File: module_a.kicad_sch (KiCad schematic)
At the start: 34 parts, among them J1 RS232, J2 Ethernet, J3 Micro_SD_Card_Det2, U1 MAX3232, U18 74LVC1G07, U2 SN74AHC123A, U3 TPD4EUSB30, U4 TPD4EUSB30, U5 TPS2553

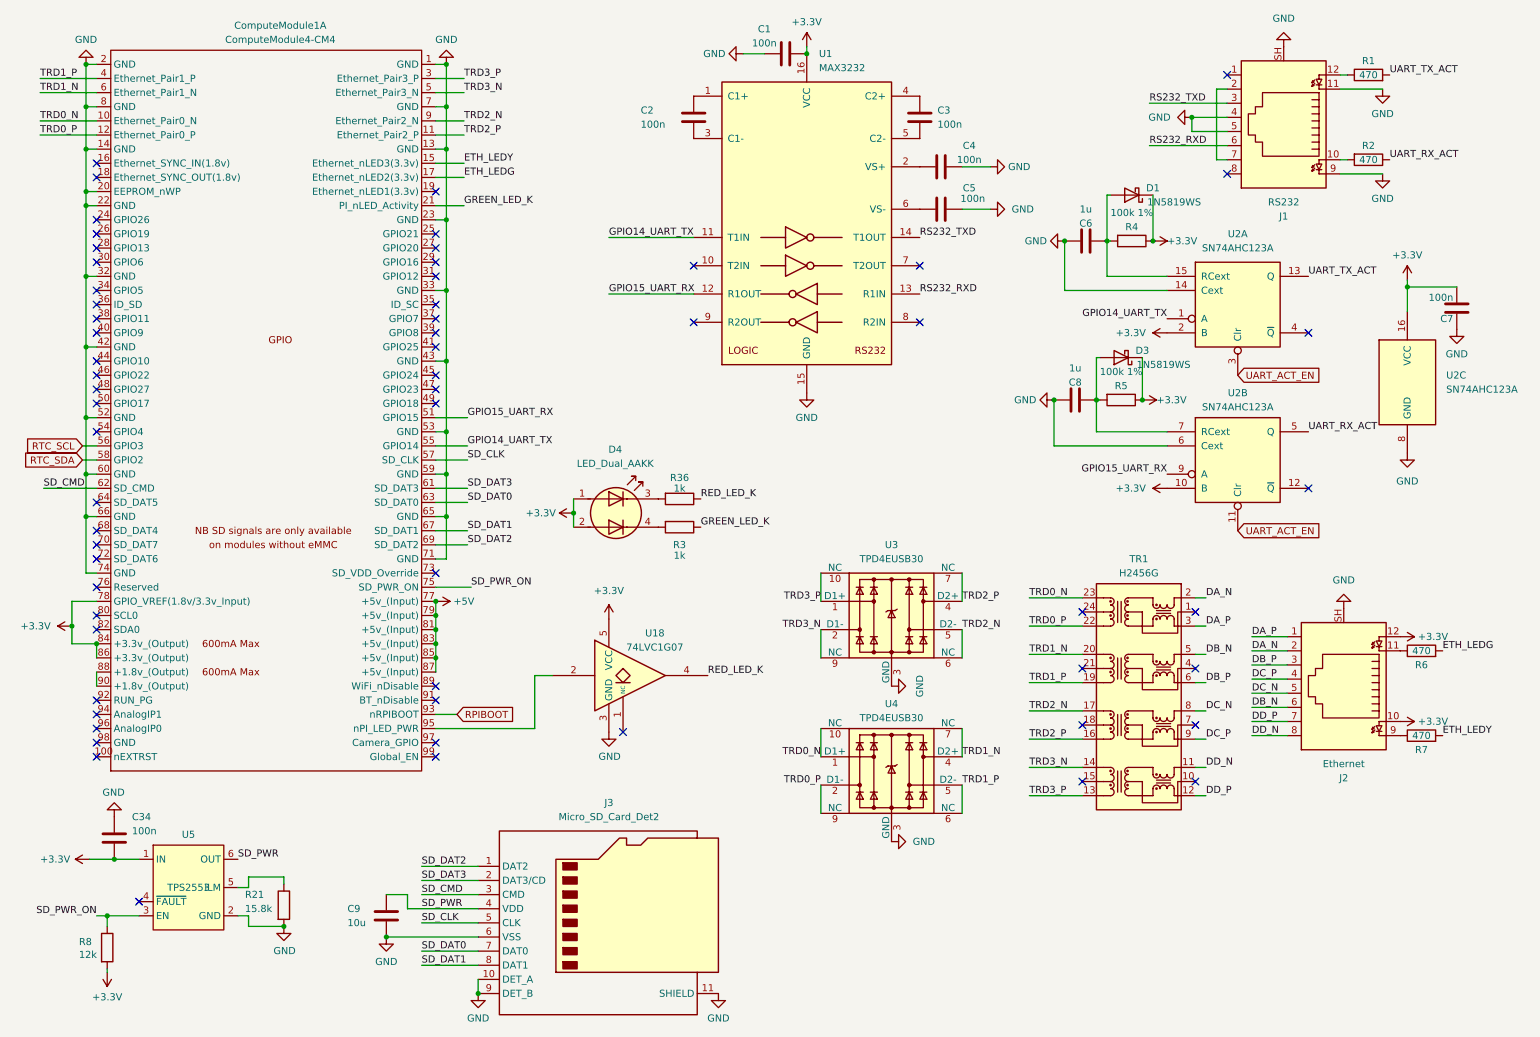
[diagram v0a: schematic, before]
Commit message: wip
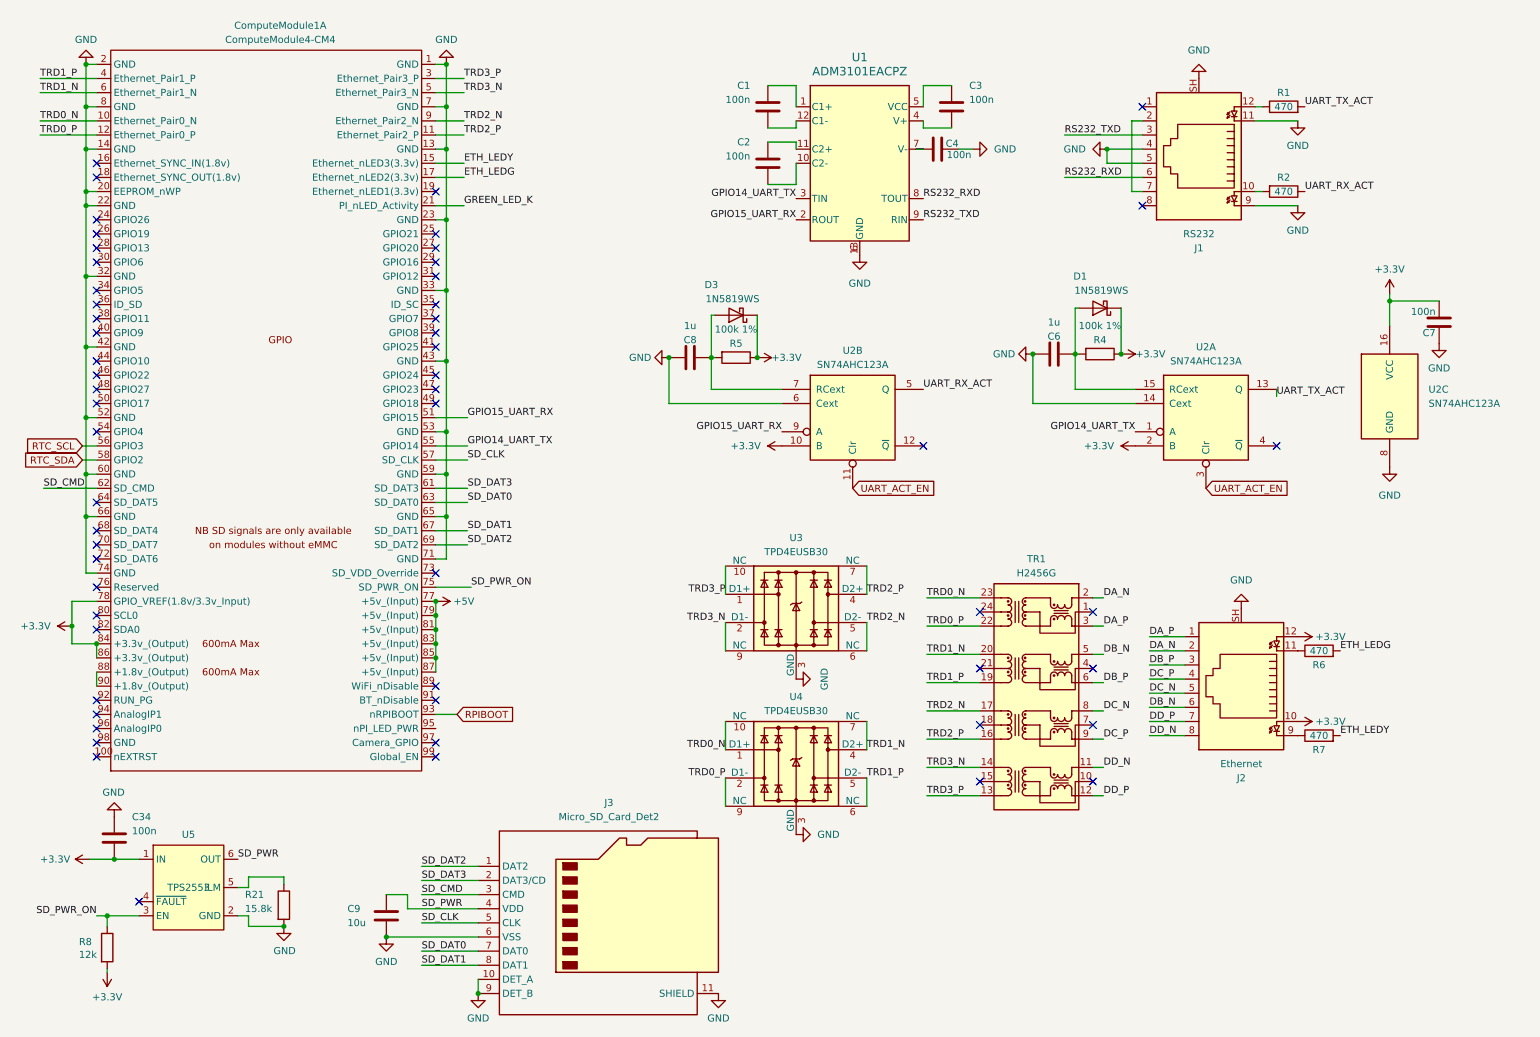
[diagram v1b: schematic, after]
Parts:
- removed C5: 100n, Capacitor_SMD:C_0402_1005Metric, symbol Device:C
- removed D4: LED_Dual_AAKK, PiCard:LED-ARRAY-SMD_4P-L3.0-W1.5-L-FD, symbol Device:LED_Dual_AAKK
- removed R3, R36: 1k, Resistor_SMD:R_0402_1005Metric, symbol Device:R
- removed U1: MAX3232, Package_SO:TSSOP-16_4.4x5mm_P0.65mm, symbol Interface_UART:MAX3232
- removed U18: 74LVC1G07, Package_TO_SOT_SMD:SOT-353_SC-70-5, symbol 74xGxx:74LVC1G07
- added U1: ADM3101EACPZ, PiCard:LFCSP-12-1EP_3x3mm_P0.5mm_EP1.3x1.3mm, symbol PiCard:ADM3101EACPZ
- U2: footprint Package_SO:TSSOP-16_4.4x5mm_P0.65mm -> Package_DFN_QFN:DHVQFN-16-1EP_2.5x3.5mm_P0.5mm_EP1x2mm
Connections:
- net +3.3V: no longer C1.2
- net GND: now also U1.13 (GND), U1.6 (GND); no longer C1.1
- net GPIO14_UART_TX: now also U1.3 (TIN)
- net GPIO15_UART_RX: now also U1.2 (ROUT)
- net RS232_RXD: now also U1.8 (TOUT)
- net RS232_TXD: now also U1.9 (RIN)
- net at C2.1: now also U1.11 (C2+)
- net at C4.1: now also U1.7 (V-)
- net at C2.2: now also U1.10 (C2-)
- net at C3.1: now also U1.5 (VCC)
- net at C3.2: now also U1.4 (V+)
- new net: C1.1, U1.1 (C1+)
- new net: C1.2, U1.12 (C1-)
- no-connect marks 62 -> 57
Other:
- moved on the sheet: C6, C7, C8, D1, D3, J1, J2, R1, R2, R4, R5, R6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
